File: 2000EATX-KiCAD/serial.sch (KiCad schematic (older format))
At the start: 52 parts, among them CN305 DB25_Stack_FemaleAndMale, CN306 POWER LED, Q300 MMBT3904, Q302 MMBT3906, U301 8520, U302 74LS32, U303 74LS08, U304 SN75188DR, U305 SN75189DR, U805 LM339

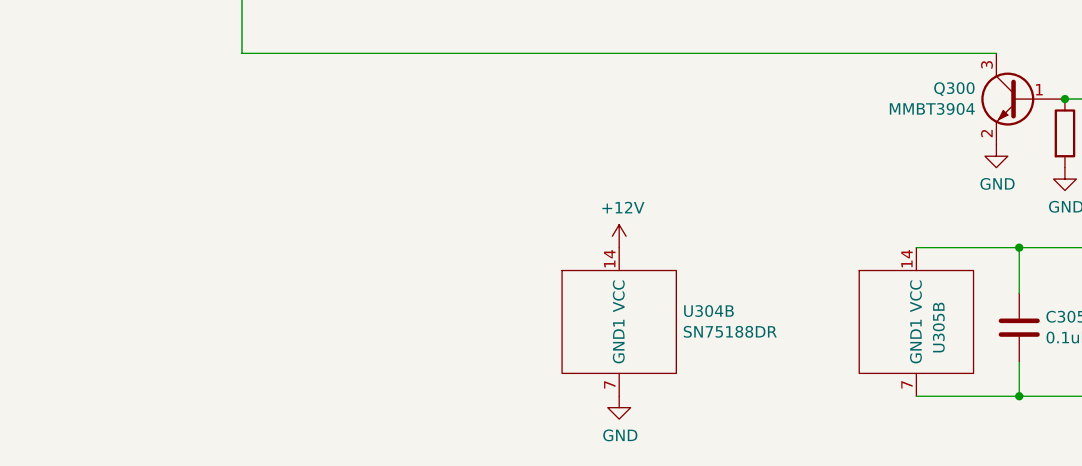
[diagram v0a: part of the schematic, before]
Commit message: Add files via upload
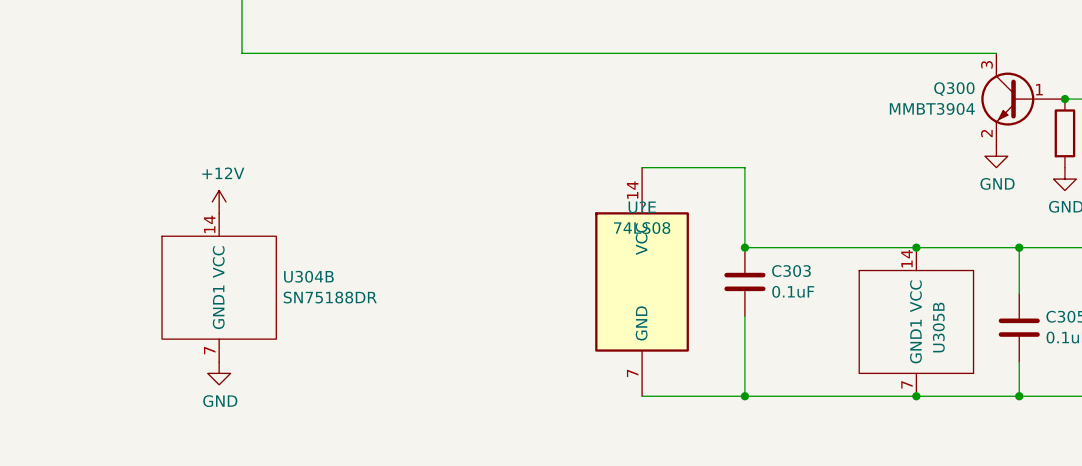
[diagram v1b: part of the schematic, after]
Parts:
- added C303: 0.1uF, Capacitor_SMD:C_1206_3216Metric, symbol Device:C
- added U?: 74LS08, symbol 74xx:74LS08
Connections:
- net +5V: now also C303.1, U?.14 (VCC)
- net GND: now also C303.2, U?.7 (GND)
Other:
- moved on the sheet: U304B
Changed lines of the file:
@@
 L Amiga-Library:SN75188DR U304
 U 2 1 6066C22E
-P 8100 9900
-F 0 "U304" H 8378 9921 50  0000 L CNN
-F 1 "SN75188DR" H 8378 9830 50  0000 L CNN
-F 2 "Package_SO:SOIC-14_3.9x8.7mm_P1.27mm" H 8050 9050 50  0001 C CNN
-F 3 "https://www.ti.com/lit/ds/symlink/mc1488.pdf?HQS=dis-dk-null-digikeymode-dsf-pf-null-wwe&ts=1616552868480" H 8100 9100 50  0001 C CNN
-	2    8100 9900
+P 6350 9750
+F 0 "U304" H 6628 9771 50  0000 L CNN
+F 1 "SN75188DR" H 6628 9680 50  0000 L CNN
+F 2 "Package_SO:SOIC-14_3.9x8.7mm_P1.27mm" H 6300 8900 50  0001 C CNN
+F 3 "https://www.ti.com/lit/ds/symlink/mc1488.pdf?HQS=dis-dk-null-digikeymode-dsf-pf-null-wwe&ts=1616552868480" H 6350 8950 50  0001 C CNN
+	2    6350 9750
 	1    0    0    -1
 $EndComp
@@
 L power:+12V #PWR0297
 U 1 1 60673697
-P 8100 9600
-F 0 "#PWR0297" H 8100 9450 50  0001 C CNN
-F 1 "+12V" H 8115 9773 50  0000 C CNN
-F 2 "" H 8100 9600 50  0001 C CNN
-F 3 "" H 8100 9600 50  0001 C CNN
-	1    8100 9600
+P 6350 9450
+F 0 "#PWR0297" H 6350 9300 50  0001 C CNN
+F 1 "+12V" H 6365 9623 50  0000 C CNN
+F 2 "" H 6350 9450 50  0001 C CNN
+F 3 "" H 6350 9450 50  0001 C CNN
+	1    6350 9450
 	1    0    0    -1
 $EndComp
@@
 L power:GND #PWR0298
 U 1 1 6067399F
-P 8100 10250
-F 0 "#PWR0298" H 8100 10000 50  0001 C CNN
-F 1 "GND" H 8105 10077 50  0000 C CNN
-F 2 "" H 8100 10250 50  0001 C CNN
-F 3 "" H 8100 10250 50  0001 C CNN
-	1    8100 10250
+P 6350 10100
+F 0 "#PWR0298" H 6350 9850 50  0001 C CNN
+F 1 "GND" H 6355 9927 50  0000 C CNN
+F 2 "" H 6350 10100 50  0001 C CNN
+F 3 "" H 6350 10100 50  0001 C CNN
+	1    6350 10100
 	1    0    0    -1
 $EndComp
@@
 	-1   0    0    1
 $EndComp
+$Comp
+L 74xx:74LS08 U?
+U 5 1 60A7C756
+P 8200 9750
+F 0 "U?" H 8200 10075 50  0000 C CNN
+F 1 "74LS08" H 8200 9984 50  0000 C CNN
+F 2 "" H 8200 9750 50  0001 C CNN
+F 3 "http://www.ti.com/lit/gpn/sn74LS08" H 8200 9750 50  0001 C CNN
+	5    8200 9750
+	1    0    0    -1
+$EndComp
+$Comp
+L Device:C C303
+U 1 1 60A965B1
+P 8650 9750
+F 0 "C303" H 8765 9796 50  0000 L CNN
+F 1 "0.1uF" H 8765 9705 50  0000 L CNN
+F 2 "Capacitor_SMD:C_1206_3216Metric" H 8688 9600 50  0001 C CNN
+F 3 "~" H 8650 9750 50  0001 C CNN
+	1    8650 9750
+	1    0    0    -1
+$EndComp
+Wire Wire Line
+	9400 9600 8650 9600
+Connection ~ 9400 9600
+Wire Wire Line
+	8200 9250 8650 9250
+Wire Wire Line
+	8650 9250 8650 9600
+Connection ~ 8650 9600
+Wire Wire Line
+	9400 10250 8650 10250
+Connection ~ 9400 10250
+Wire Wire Line
+	8650 9900 8650 10250
+Connection ~ 8650 10250
+Wire Wire Line
+	8650 10250 8200 10250
 $EndSCHEMATC

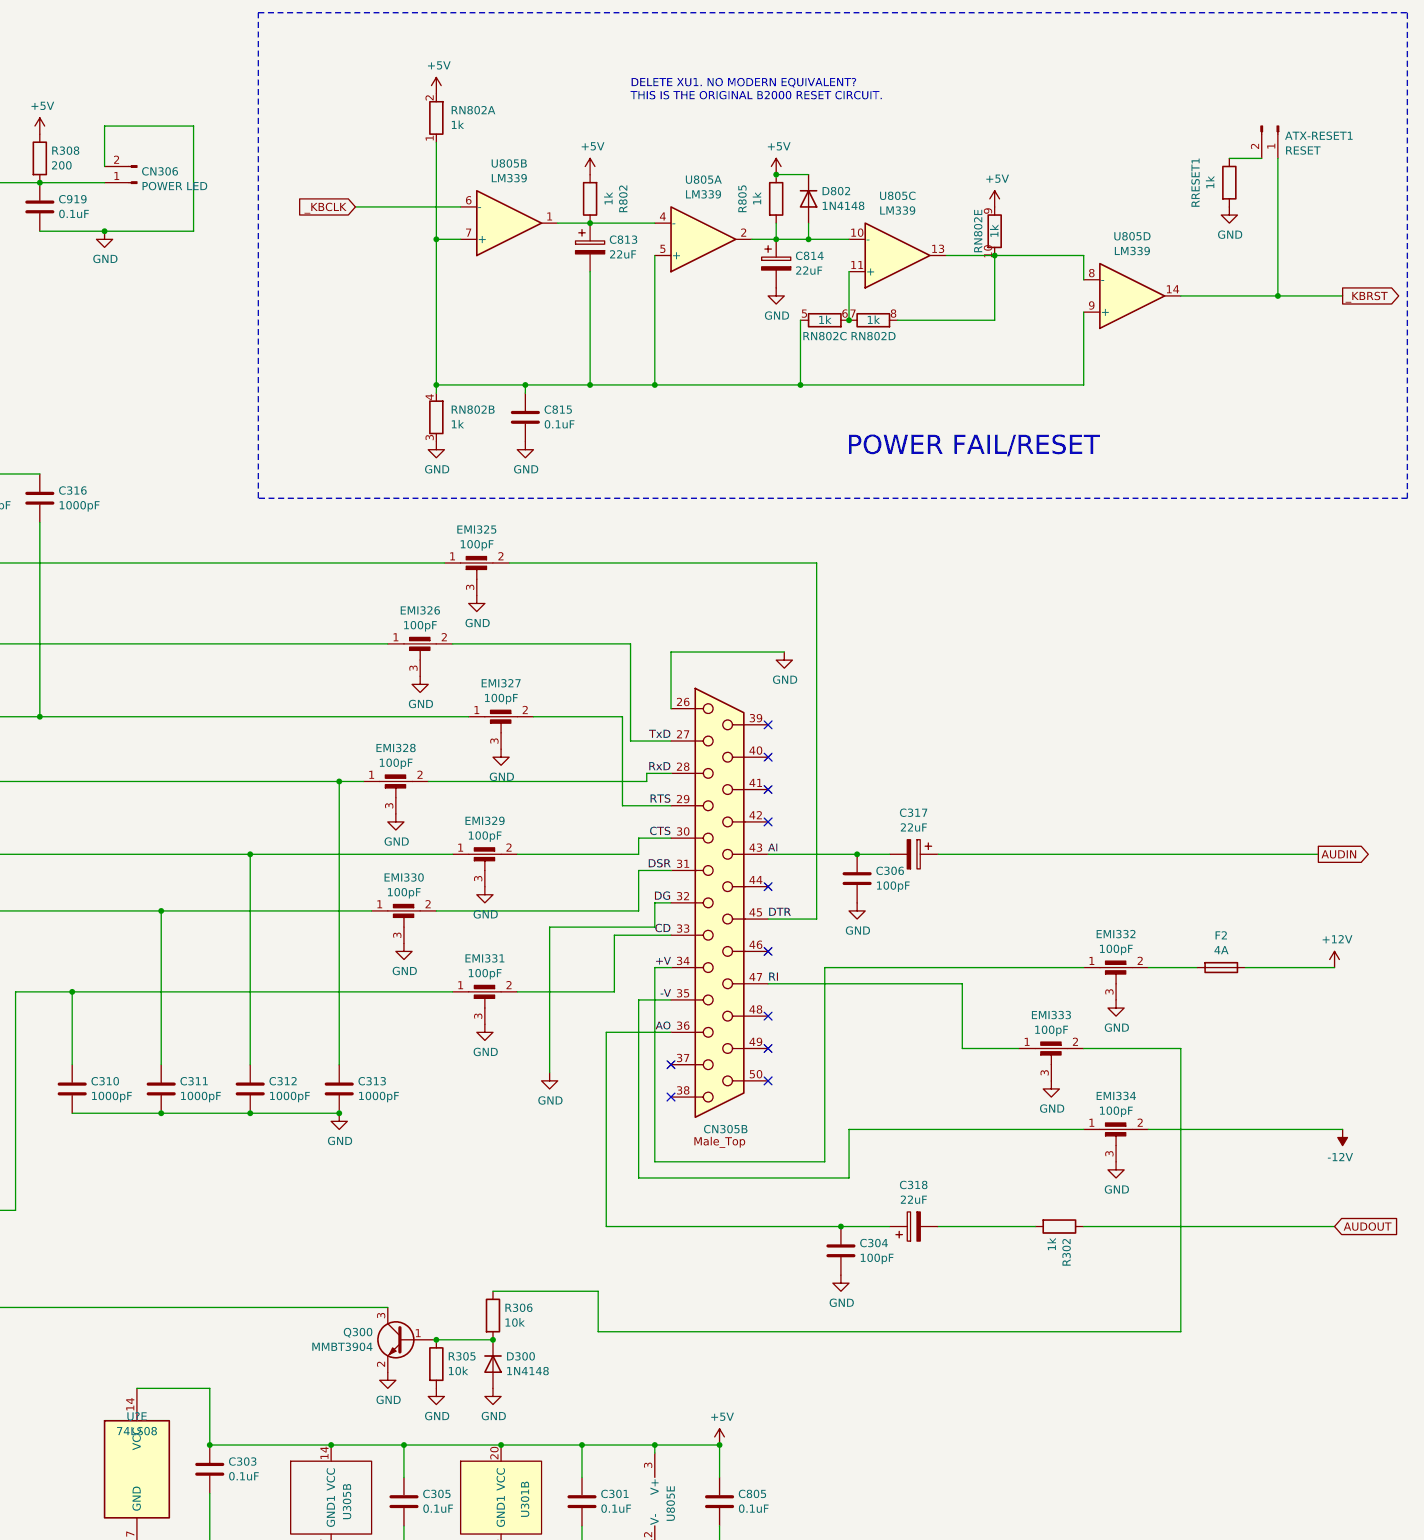
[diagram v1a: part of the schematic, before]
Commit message: Add files via upload
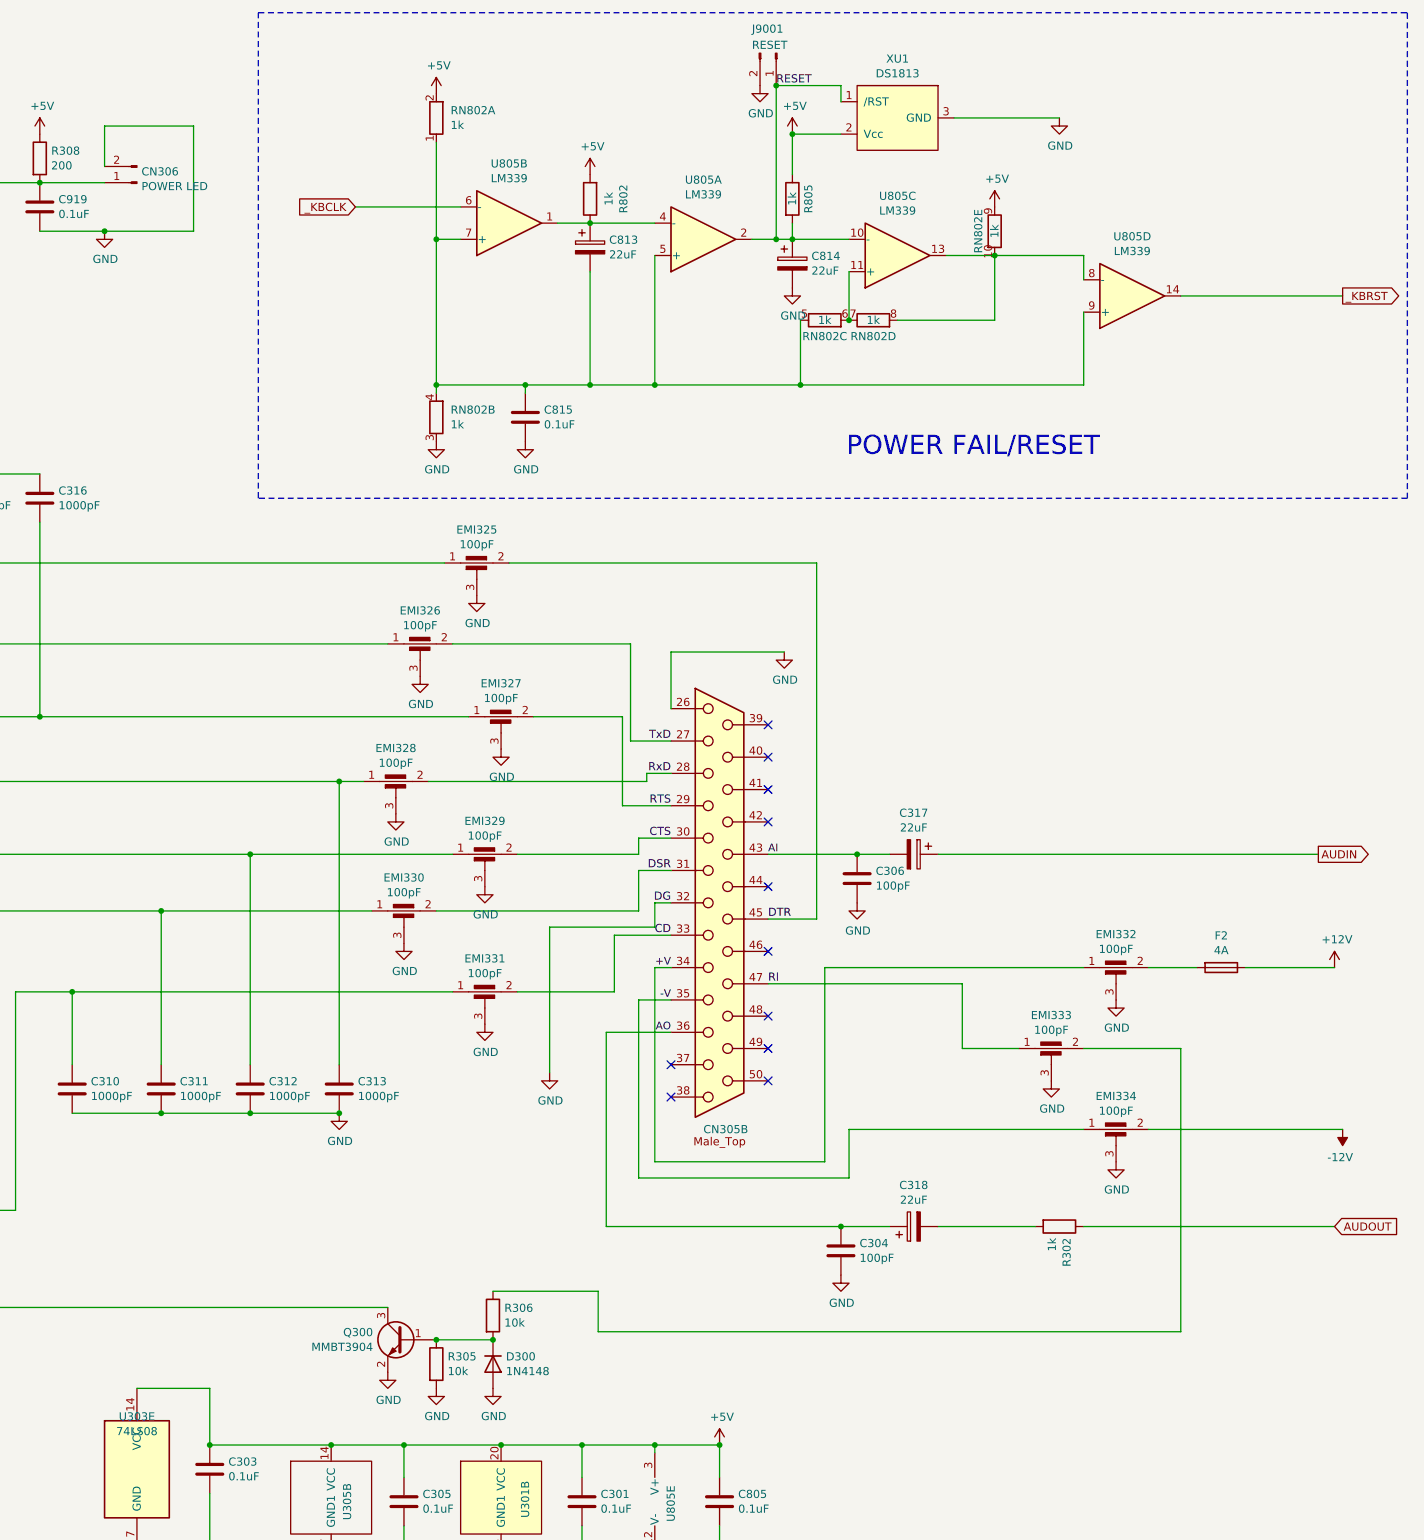
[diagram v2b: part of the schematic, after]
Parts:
- removed D802: 1N4148, Diode_SMD:D_SOD-323, symbol Diode:1N4148
- removed RRESET1: 1k, Resistor_SMD:R_1206_3216Metric, symbol Device:R
- added XU1: DS1813, Package_TO_SOT_SMD:SOT-23, symbol Amiga-Library:DS1813
- gave numbers to parts that had none: 1
- renumbered ATX-RESET1 to J9001
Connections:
- net +5V: now also XU1.2 (Vcc)
- net GND: now also J9001.2 (Pin_2), XU1.3 (GND)
- net _KBRST: no longer J9001.1 (Pin_1)
- net RESET: now reaches C814.1, R805.2, U805.10 (-), U805.2
- net RESET: now also J9001.1 (Pin_1), XU1.1 (/RST)
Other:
- note removed: "DELETE XU1. NO MODERN EQUIVALENT?\nTHIS IS THE ORIGINAL B2000 RESET CIRCUIT."
- moved on the sheet: C814, J9001, R805
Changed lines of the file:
@@
 Wire Wire Line
 	12000 2150 12150 2150
-$Comp
-L Diode:1N4148 D802
-U 1 1 609295DA
-P 12350 1900
-F 0 "D802" V 12304 1980 50  0000 L CNN
-F 1 "1N4148" V 12395 1980 50  0000 L CNN
-F 2 "Diode_SMD:D_SOD-323" H 12350 1725 50  0001 C CNN
-F 3 "https://assets.nexperia.com/documents/data-sheet/1N4148_1N4448.pdf" H 12350 1900 50  0001 C CNN
-F 4 "1N4148WSTR" V 12350 1900 50  0001 C CNN "pART"
-	1    12350 1900
-	0    1    1    0
-$EndComp
-Wire Wire Line
-	12350 2050 12350 2150
-Connection ~ 12350 2150
-Wire Wire Line
-	12350 2150 12600 2150
-Wire Wire Line
-	12150 2050 12150 2150
-Connection ~ 12150 2150
-Wire Wire Line
-	12150 2150 12350 2150
+Wire Wire Line
+	12250 2050 12250 2150
+Connection ~ 12250 2150
 $Comp
 L Device:R R805
 U 1 1 609496BA
-P 12150 1900
-F 0 "R805" V 11943 1900 50  0000 C CNN
-F 1 "1k" V 12034 1900 50  0000 C CNN
-F 2 "Resistor_SMD:R_1206_3216Metric" V 12080 1900 50  0001 C CNN
-F 3 "~" H 12150 1900 50  0001 C CNN
-	1    12150 1900
+P 12250 1900
+F 0 "R805" V 12350 1900 50  0000 C CNN
+F 1 "1k" V 12250 1900 50  0000 C CNN
+F 2 "Resistor_SMD:R_1206_3216Metric" V 12180 1900 50  0001 C CNN
+F 3 "~" H 12250 1900 50  0001 C CNN
+	1    12250 1900
 	1    0    0    -1
 $EndComp
@@
 L Device:CP C814
 U 1 1 60949F6D
-P 12150 2300
-F 0 "C814" H 12268 2346 50  0000 L CNN
-F 1 "22uF" H 12268 2255 50  0000 L CNN
-F 2 "Capacitor_SMD:CP_Elec_6.3x5.8" H 12188 2150 50  0001 C CNN
-F 3 "~" H 12150 2300 50  0001 C CNN
-	1    12150 2300
-	1    0    0    -1
-$EndComp
-Wire Wire Line
-	12350 1750 12150 1750
+P 12250 2300
+F 0 "C814" H 12368 2346 50  0000 L CNN
+F 1 "22uF" H 12368 2255 50  0000 L CNN
+F 2 "Capacitor_SMD:CP_Elec_6.3x5.8" H 12288 2150 50  0001 C CNN
+F 3 "~" H 12250 2300 50  0001 C CNN
+	1    12250 2300
+	1    0    0    -1
+$EndComp
 $Comp
 L power:+5V #PWR0324
 U 1 1 60957A19
-P 12150 1750
-F 0 "#PWR0324" H 12150 1600 50  0001 C CNN
-F 1 "+5V" H 12165 1923 50  0000 C CNN
-F 2 "" H 12150 1750 50  0001 C CNN
-F 3 "" H 12150 1750 50  0001 C CNN
-	1    12150 1750
-	1    0    0    -1
-$EndComp
-Connection ~ 12150 1750
-Text Notes 11250 1300 0    50   ~ 0
-DELETE XU1. NO MODERN EQUIVALENT?\nTHIS IS THE ORIGINAL B2000 RESET CIRCUIT.
+P 12250 1500
+F 0 "#PWR0324" H 12250 1350 50  0001 C CNN
+F 1 "+5V" H 12265 1673 50  0000 C CNN
+F 2 "" H 12250 1500 50  0001 C CNN
+F 3 "" H 12250 1500 50  0001 C CNN
+	1    12250 1500
+	1    0    0    -1
+$EndComp
 Wire Wire Line
 	12600 2350 12600 2650
@@
 POWER FAIL/RESET
 $Comp
-L Connector:Conn_01x02_Male ATX-RESET1
+L Connector:Conn_01x02_Male J9001
 U 1 1 60A28FC2
-P 15250 1450
-F 0 "ATX-RESET1" V 15312 1494 50  0000 L CNN
-F 1 "RESET" V 15403 1494 50  0000 L CNN
-F 2 "Connector_PinHeader_2.54mm:PinHeader_1x02_P2.54mm_Vertical" H 15250 1450 50  0001 C CNN
-F 3 "~" H 15250 1450 50  0001 C CNN
-	1    15250 1450
+P 12150 1000
+F 0 "J9001" V 12000 850 50  0000 L CNN
+F 1 "RESET" V 12100 850 50  0000 L CNN
+F 2 "Connector_PinHeader_2.54mm:PinHeader_1x02_P2.54mm_Vertical" H 12150 1000 50  0001 C CNN
+F 3 "~" H 12150 1000 50  0001 C CNN
+	1    12150 1000
 	0    1    1    0
-$EndComp
-Wire Wire Line
-	15150 1650 14950 1650
-$Comp
-L Device:R RRESET1
-U 1 1 60A56EBC
-P 14950 1800
-F 0 "RRESET1" V 14743 1800 50  0000 C CNN
-F 1 "1k" V 14834 1800 50  0000 C CNN
-F 2 "Resistor_SMD:R_1206_3216Metric" V 14880 1800 50  0001 C CNN
-F 3 "~" H 14950 1800 50  0001 C CNN
-	1    14950 1800
-	1    0    0    -1
 $EndComp
 $Comp
 L power:GND #PWR0326
 U 1 1 60A59CE8
-P 14950 1950
-F 0 "#PWR0326" H 14950 1700 50  0001 C CNN
-F 1 "GND" H 14955 1777 50  0000 C CNN
-F 2 "" H 14950 1950 50  0001 C CNN
-F 3 "" H 14950 1950 50  0001 C CNN
-	1    14950 1950
-	1    0    0    -1
-$EndComp
-Wire Wire Line
-	14650 2500 15250 2500
-Wire Wire Line
-	15250 1650 15250 2500
-Connection ~ 15250 2500
-Wire Wire Line
-	15250 2500 15650 2500
+P 13900 1400
+F 0 "#PWR0326" H 13900 1150 50  0001 C CNN
+F 1 "GND" H 13905 1227 50  0000 C CNN
+F 2 "" H 13900 1400 50  0001 C CNN
+F 3 "" H 13900 1400 50  0001 C CNN
+	1    13900 1400
+	1    0    0    -1
+$EndComp
 $Comp
 L power:GND #PWR0327
 U 1 1 60A7BF0B
-P 12150 2450
-F 0 "#PWR0327" H 12150 2200 50  0001 C CNN
-F 1 "GND" H 12155 2277 50  0000 C CNN
-F 2 "" H 12150 2450 50  0001 C CNN
-F 3 "" H 12150 2450 50  0001 C CNN
-	1    12150 2450
+P 12250 2450
+F 0 "#PWR0327" H 12250 2200 50  0001 C CNN
+F 1 "GND" H 12255 2277 50  0000 C CNN
+F 2 "" H 12250 2450 50  0001 C CNN
+F 3 "" H 12250 2450 50  0001 C CNN
+	1    12250 2450
 	1    0    0    -1
 $EndComp
@@
 $EndComp
 $Comp
-L 74xx:74LS08 U?
+L 74xx:74LS08 U303
 U 5 1 60A7C756
 P 8200 9750
-F 0 "U?" H 8200 10075 50  0000 C CNN
+F 0 "U303" H 8200 10075 50  0000 C CNN
 F 1 "74LS08" H 8200 9984 50  0000 C CNN
 F 2 "" H 8200 9750 50  0001 C CNN
@@
 Wire Wire Line
 	8650 10250 8200 10250
+$Comp
+L Amiga-Library:DS1813 XU1
+U 1 1 607B0B2C
+P 13000 1400
+F 0 "XU1" V 12635 1300 50  0000 C CNN
+F 1 "DS1813" V 12726 1300 50  0000 C CNN
+F 2 "Package_TO_SOT_SMD:SOT-23" H 13000 1400 50  0001 C CNN
+F 3 "" H 13000 1400 50  0001 C CNN
+	1    13000 1400
+	0    1    1    0
+$EndComp
+Wire Wire Line
+	14650 2500 15650 2500
+Wire Wire Line
+	12250 2150 12600 2150
+Wire Wire Line
+	12550 1500 12250 1500
+Wire Wire Line
+	12250 1500 12250 1750
+Connection ~ 12250 1500
+Wire Wire Line
+	13250 1400 13900 1400
+Wire Wire Line
+	12550 1300 12550 1200
+Wire Wire Line
+	12550 1200 12150 1200
+Wire Wire Line
+	12150 1200 12150 2150
+Connection ~ 12150 2150
+Wire Wire Line
+	12150 2150 12250 2150
+Connection ~ 12150 1200
+$Comp
+L power:GND #PWR0176
+U 1 1 6083E71B
+P 12050 1200
+F 0 "#PWR0176" H 12050 950 50  0001 C CNN
+F 1 "GND" H 12055 1027 50  0000 C CNN
+F 2 "" H 12050 1200 50  0001 C CNN
+F 3 "" H 12050 1200 50  0001 C CNN
+	1    12050 1200
+	1    0    0    -1
+$EndComp
+Text Label 12150 1200 0    50   ~ 0
+RESET
 $EndSCHEMATC
